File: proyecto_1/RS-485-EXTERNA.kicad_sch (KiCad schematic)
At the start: 0 parts

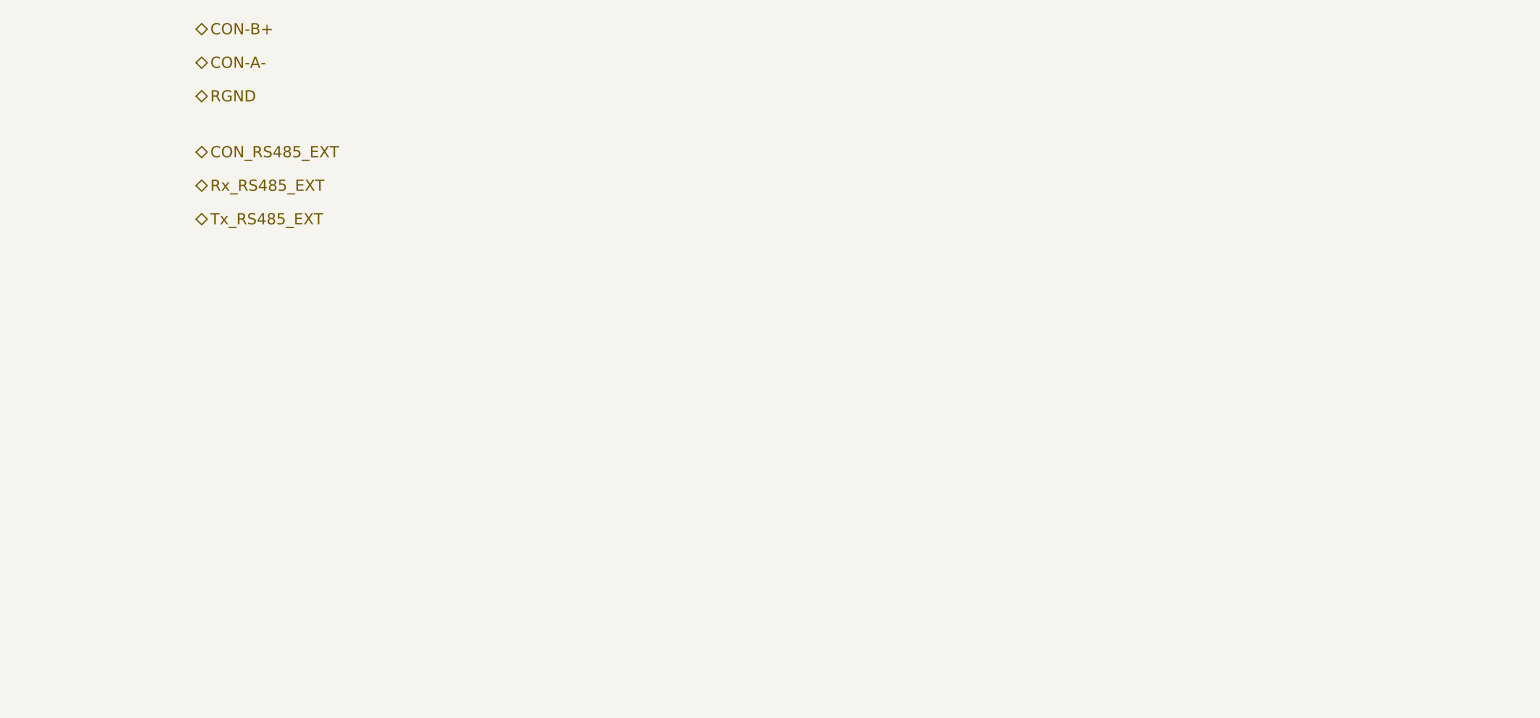
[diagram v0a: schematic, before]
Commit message: nuevos circuitos de pcb
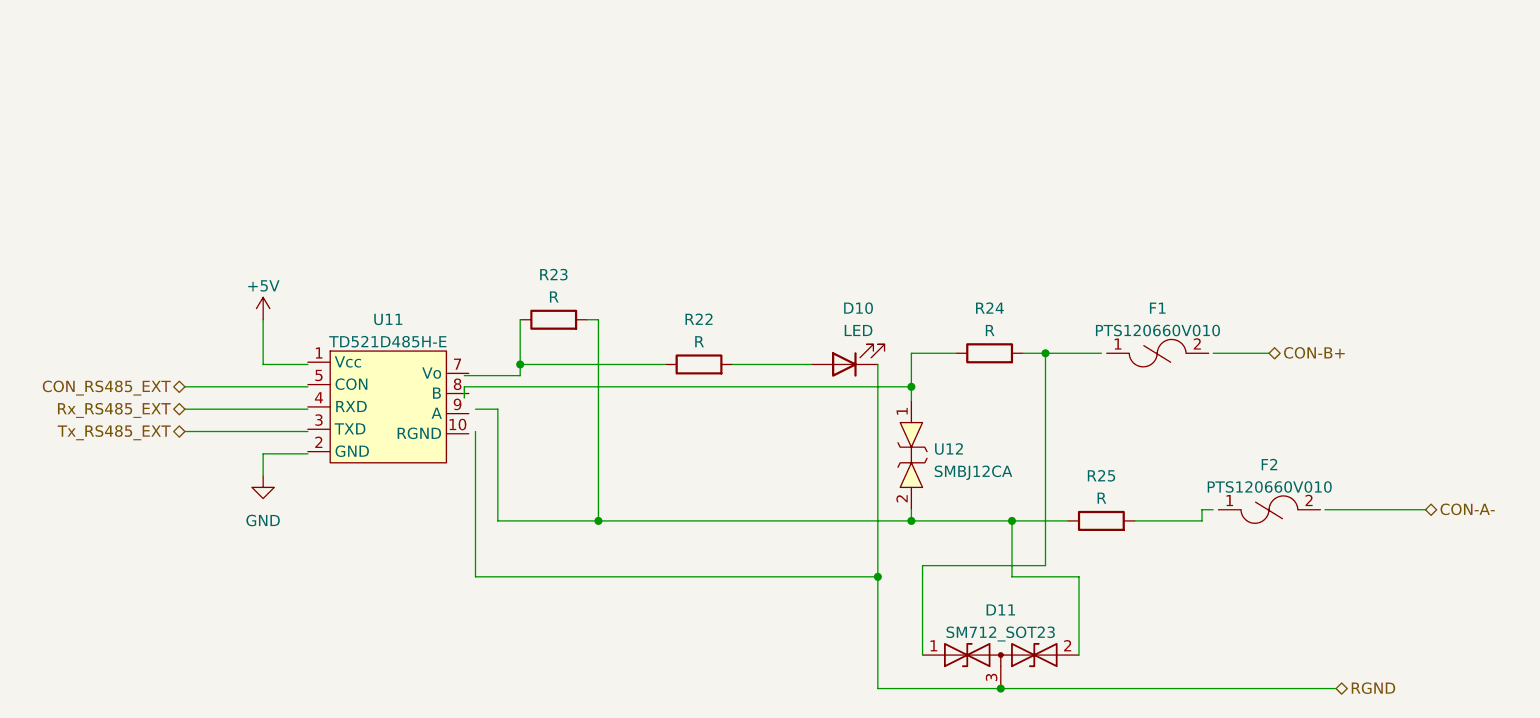
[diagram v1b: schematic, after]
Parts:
- added D10: LED, symbol Device:LED
- added D11: SM712_SOT23, Package_TO_SOT_SMD:SOT-23, symbol Diode:SM712_SOT23
- added F1, F2: PTS120660V010, Nueva carpeta:RESC3115X65N, symbol nuevo simbolos:PTS120660V010
- added R22, R23, R24, R25: R, symbol Device:R
- added U11: TD521D485H-E, nuevo simbolo:TD521D485H-E, symbol nuevo simbolos:TD521D485H-E
- added U12: SMBJ12CA, nuevo simbolo:SMBJ12CA, symbol nuevo simbolos:SMBJ12CA
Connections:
- net RGND: now also D10.1 (K), D11.3 (common)
- new net: R22.1, R23.1
- new net: D10.2 (A), R22.2
- new net: D11.2 (A2), R23.2, R25.1, U12.2
- new net: D11.1 (A1), R24.2
- new net: R24.1, U12.1

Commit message: agregados al esquematico
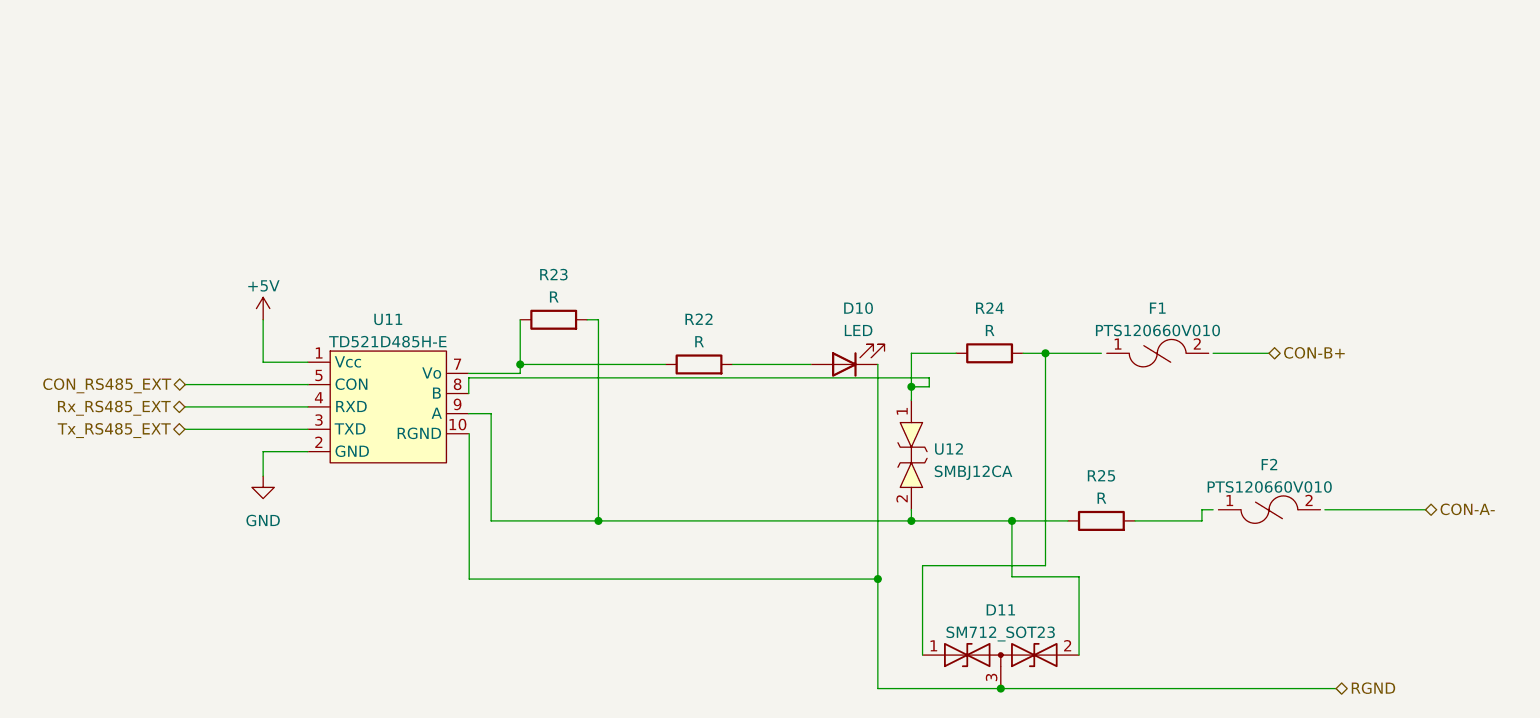
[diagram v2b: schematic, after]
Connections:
- net +5V: now also U11.1 (Vcc)
- net GND: now also U11.2 (GND)
- net Rx_RS485_EXT: now also U11.4 (RXD)
- net Tx_RS485_EXT: now also U11.3 (TXD)
- net at R22.1, R23.1: now also U11.7 (Vo)
- net at D11.2 (A2), R23.2, R25.1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: now also U11.9 (A)
- net at U11.8 (B): now also R24.1, U12.1
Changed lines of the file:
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@@
 (kicad_sch (version 20230121) (generator eeschema)
   (paper "A4")
-  (junction (at 173.99 111.76) (diameter 0) (color 0 0 0 0)
-  )
   (junction (at 142.24 105.41) (diameter 0) (color 0 0 0 0)
   )
   (junction (at 133.35 87.63) (diameter 0) (color 0 0 0 0)
+  )
+  (junction (at 173.99 112.014) (diameter 0) (color 0 0 0 0)
   )
   (junction (at 193.04 86.36) (diameter 0) (color 0 0 0 0)
@@
     (stroke (width 0) (type default))
   )
+  (wire (pts (xy 173.99 87.63) (xy 173.99 112.014))
+    (stroke (width 0) (type default))
+  )
   (wire (pts (xy 189.23 111.76) (xy 189.23 105.41))
     (stroke (width 0) (type default))
   )
-  (wire (pts (xy 127 90.17) (xy 177.8 90.17))
+  (wire (pts (xy 127.508 89.154) (xy 179.832 89.154))
     (stroke (width 0) (type default))
   )
-  (wire (pts (xy 95.25 90.17) (xy 109.22 90.17))
+  (wire (pts (xy 95.3008 89.916) (xy 109.2708 89.916))
     (stroke (width 0) (type default))
   )
@@
     (stroke (width 0) (type default))
   )
-  (wire (pts (xy 127 88.9) (xy 133.35 88.9))
+  (wire (pts (xy 127.508 88.646) (xy 133.35 88.646))
     (stroke (width 0) (type default))
   )
@@
     (stroke (width 0) (type default))
   )
-  (wire (pts (xy 128.27 95.25) (xy 128.27 111.76))
+  (wire (pts (xy 127.5588 95.504) (xy 127.5588 112.014))
     (stroke (width 0) (type default))
   )
-  (wire (pts (xy 109.22 97.79) (xy 104.14 97.79))
+  (wire (pts (xy 179.832 89.154) (xy 179.832 90.17))
+    (stroke (width 0) (type default))
+  )
+  (wire (pts (xy 109.22 97.536) (xy 104.14 97.536))
     (stroke (width 0) (type default))
   )
@@
     (stroke (width 0) (type default))
   )
-  (wire (pts (xy 95.25 95.25) (xy 109.22 95.25))
+  (wire (pts (xy 95.25 94.996) (xy 109.22 94.996))
     (stroke (width 0) (type default))
   )
-  (wire (pts (xy 127 90.17) (xy 127 91.44))
+  (wire (pts (xy 127.508 89.154) (xy 127.508 90.932))
     (stroke (width 0) (type default))
   )
@@
     (stroke (width 0) (type default))
   )
-  (wire (pts (xy 109.22 87.63) (xy 104.14 87.63))
+  (wire (pts (xy 109.22 87.376) (xy 104.14 87.376))
     (stroke (width 0) (type default))
   )
@@
     (stroke (width 0) (type default))
   )
-  (wire (pts (xy 128.27 111.76) (xy 173.99 111.76))
+  (wire (pts (xy 127.5588 112.014) (xy 173.99 112.014))
     (stroke (width 0) (type default))
   )
@@
     (stroke (width 0) (type default))
   )
-  (wire (pts (xy 133.35 87.63) (xy 133.35 88.9))
+  (wire (pts (xy 133.35 87.63) (xy 133.35 88.646))
     (stroke (width 0) (type default))
   )
@@
     (stroke (width 0) (type default))
   )
-  (wire (pts (xy 104.14 87.63) (xy 104.14 82.55))
+  (wire (pts (xy 104.14 87.376) (xy 104.14 82.55))
     (stroke (width 0) (type default))
   )
-  (wire (pts (xy 130.81 105.41) (xy 142.24 105.41))
+  (wire (pts (xy 130.048 105.41) (xy 142.24 105.41))
     (stroke (width 0) (type default))
   )
-  (wire (pts (xy 95.25 92.71) (xy 109.22 92.71))
+  (wire (pts (xy 95.25 92.456) (xy 109.22 92.456))
     (stroke (width 0) (type default))
   )
@@
     (stroke (width 0) (type default))
   )
-  (wire (pts (xy 104.14 97.79) (xy 104.14 100.33))
+  (wire (pts (xy 104.14 97.536) (xy 104.14 100.33))
     (stroke (width 0) (type default))
   )
-  (wire (pts (xy 128.27 92.71) (xy 130.81 92.71))
+  (wire (pts (xy 127.508 93.218) (xy 130.048 93.218))
     (stroke (width 0) (type default))
   )
-  (wire (pts (xy 173.99 87.63) (xy 173.99 111.76))
-    (stroke (width 0) (type default))
-  )
-  (wire (pts (xy 173.99 124.46) (xy 173.99 111.76))
+  (wire (pts (xy 173.99 124.46) (xy 173.99 112.014))
     (stroke (width 0) (type default))
   )
@@
     (stroke (width 0) (type default))
   )
-  (wire (pts (xy 130.81 105.41) (xy 130.81 92.71))
+  (wire (pts (xy 130.048 105.41) (xy 130.048 93.218))
+    (stroke (width 0) (type default))
+  )
+  (wire (pts (xy 179.832 90.17) (xy 177.8 90.17))
     (stroke (width 0) (type default))
   )
@@
     (effects (font (size 1.27 1.27)) (justify left))
   )
-  (hierarchical_label "Rx_RS485_EXT" (shape bidirectional) (at 95.25 92.71 180) (fields_autoplaced)
+  (hierarchical_label "Rx_RS485_EXT" (shape bidirectional) (at 95.25 92.456 180) (fields_autoplaced)
     (effects (font (size 1.27 1.27)) (justify right))
   )
@@
     (effects (font (size 1.27 1.27)) (justify left))
   )
-  (hierarchical_label "CON_RS485_EXT" (shape bidirectional) (at 95.25 90.17 180) (fields_autoplaced)
+  (hierarchical_label "CON_RS485_EXT" (shape bidirectional) (at 95.3008 89.916 180) (fields_autoplaced)
     (effects (font (size 1.27 1.27)) (justify right))
   )
-  (hierarchical_label "Tx_RS485_EXT" (shape bidirectional) (at 95.25 95.25 180) (fields_autoplaced)
+  (hierarchical_label "Tx_RS485_EXT" (shape bidirectional) (at 95.25 94.996 180) (fields_autoplaced)
     (effects (font (size 1.27 1.27)) (justify right))
   )

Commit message: avance del proyecto
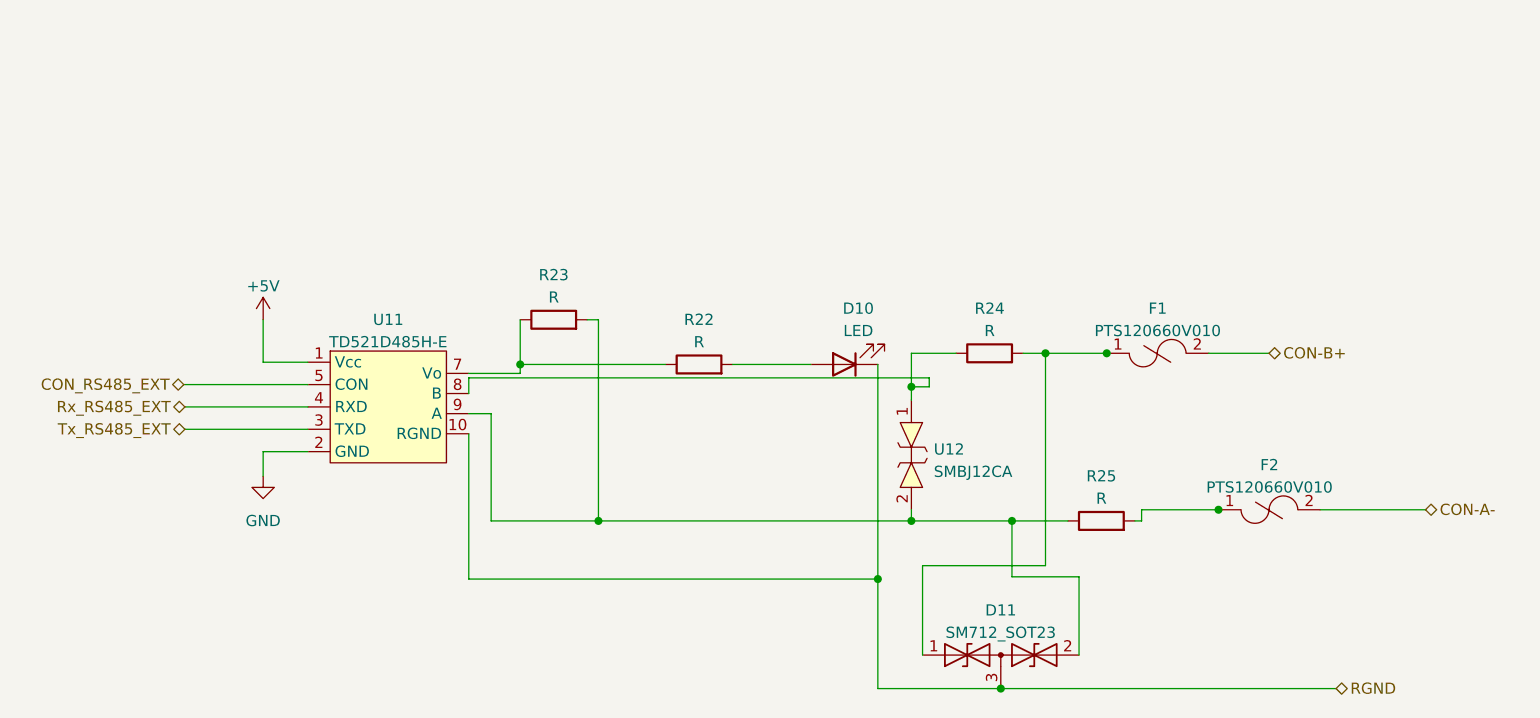
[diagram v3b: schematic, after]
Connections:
- net CON-A-: now also F2.2
- net CON-B+: now also F1.2
- net CON_RS485_EXT: now also U11.5 (CON)
- net RGND: now also U11.10 (RGND)
- net at F2.1: now also R25.2
- net at D11.1 (A1), R24.2: now also F1.1
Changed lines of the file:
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@@
 (kicad_sch (version 20230121) (generator eeschema)
   (paper "A4")
+  (junction (at 193.04 86.36) (diameter 0) (color 0 0 0 0)
+  )
   (junction (at 142.24 105.41) (diameter 0) (color 0 0 0 0)
   )
@@
   (junction (at 173.99 112.014) (diameter 0) (color 0 0 0 0)
   )
-  (junction (at 193.04 86.36) (diameter 0) (color 0 0 0 0)
+  (junction (at 189.23 105.41) (diameter 0) (color 0 0 0 0)
   )
-  (junction (at 189.23 105.41) (diameter 0) (color 0 0 0 0)
+  (junction (at 212.6996 104.14) (diameter 0) (color 0 0 0 0)
   )
   (junction (at 177.8 105.41) (diameter 0) (color 0 0 0 0)
@@
   (junction (at 187.96 124.46) (diameter 0) (color 0 0 0 0)
   )
-  (wire (pts (xy 224.79 104.14) (xy 236.22 104.14))
+  (junction (at 199.9996 86.36) (diameter 0) (color 0 0 0 0)
+  )
+  (wire (pts (xy 95.123 89.916) (xy 109.22 89.916))
     (stroke (width 0) (type default))
   )
@@
     (stroke (width 0) (type default))
   )
-  (wire (pts (xy 95.3008 89.916) (xy 109.2708 89.916))
-    (stroke (width 0) (type default))
-  )
   (wire (pts (xy 177.8 90.17) (xy 177.8 91.694))
     (stroke (width 0) (type default))
   )
   (wire (pts (xy 193.04 110.49) (xy 193.04 86.36))
+    (stroke (width 0) (type default))
+  )
+  (wire (pts (xy 127.508 95.504) (xy 127.508 112.014))
     (stroke (width 0) (type default))
   )
@@
     (stroke (width 0) (type default))
   )
-  (wire (pts (xy 127.5588 95.504) (xy 127.5588 112.014))
+  (wire (pts (xy 203.962 104.14) (xy 212.6996 104.14))
     (stroke (width 0) (type default))
   )
   (wire (pts (xy 179.832 89.154) (xy 179.832 90.17))
+    (stroke (width 0) (type default))
+  )
+  (wire (pts (xy 224.282 104.14) (xy 236.22 104.14))
     (stroke (width 0) (type default))
   )
@@
     (stroke (width 0) (type default))
   )
-  (wire (pts (xy 212.09 86.36) (xy 218.44 86.36))
-    (stroke (width 0) (type default))
-  )
   (wire (pts (xy 187.96 124.46) (xy 226.06 124.46))
     (stroke (width 0) (type default))
   )
-  (wire (pts (xy 127.5588 112.014) (xy 173.99 112.014))
+  (wire (pts (xy 193.04 86.36) (xy 199.9996 86.36))
     (stroke (width 0) (type default))
   )
@@
     (stroke (width 0) (type default))
   )
-  (wire (pts (xy 193.04 86.36) (xy 199.39 86.36))
-    (stroke (width 0) (type default))
-  )
   (wire (pts (xy 196.85 120.65) (xy 196.85 111.76))
     (stroke (width 0) (type default))
   )
-  (wire (pts (xy 210.82 104.14) (xy 212.09 104.14))
+  (wire (pts (xy 127.508 112.014) (xy 173.99 112.014))
     (stroke (width 0) (type default))
   )
@@
     (stroke (width 0) (type default))
   )
-  (wire (pts (xy 177.8 105.41) (xy 189.23 105.41))
+  (wire (pts (xy 203.962 105.41) (xy 203.2 105.41))
     (stroke (width 0) (type default))
   )
-  (wire (pts (xy 203.2 105.41) (xy 210.82 105.41))
+  (wire (pts (xy 177.8 105.41) (xy 189.23 105.41))
     (stroke (width 0) (type default))
   )
@@
     (stroke (width 0) (type default))
   )
-  (wire (pts (xy 173.99 124.46) (xy 173.99 112.014))
+  (wire (pts (xy 211.582 86.36) (xy 218.44 86.36))
+    (stroke (width 0) (type default))
+  )
+  (wire (pts (xy 212.6996 104.14) (xy 212.725 104.14))
     (stroke (width 0) (type default))
   )
@@
     (stroke (width 0) (type default))
   )
-  (wire (pts (xy 210.82 105.41) (xy 210.82 104.14))
+  (wire (pts (xy 173.99 124.46) (xy 187.96 124.46))
     (stroke (width 0) (type default))
   )
-  (wire (pts (xy 173.99 124.46) (xy 187.96 124.46))
+  (wire (pts (xy 199.9996 86.36) (xy 200.025 86.36))
+    (stroke (width 0) (type default))
+  )
+  (wire (pts (xy 203.962 104.14) (xy 203.962 105.41))
     (stroke (width 0) (type default))
   )
@@
   )
   (wire (pts (xy 179.832 90.17) (xy 177.8 90.17))
+    (stroke (width 0) (type default))
+  )
+  (wire (pts (xy 173.99 112.014) (xy 173.99 124.46))
     (stroke (width 0) (type default))
   )
@@
     (effects (font (size 1.27 1.27)) (justify left))
   )
-  (hierarchical_label "CON_RS485_EXT" (shape bidirectional) (at 95.3008 89.916 180) (fields_autoplaced)
+  (hierarchical_label "CON_RS485_EXT" (shape bidirectional) (at 95.123 89.916 180) (fields_autoplaced)
     (effects (font (size 1.27 1.27)) (justify right))
   )
